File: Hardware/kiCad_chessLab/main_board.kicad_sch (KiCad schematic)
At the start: 23 parts, among them IC4 ESP32-C6-WROOM-1-N8, J4 TYPE-C-31-M-12, J5 DATA, J6 PWR, SW2 RST, SW3 BOOT, U3 74HC138

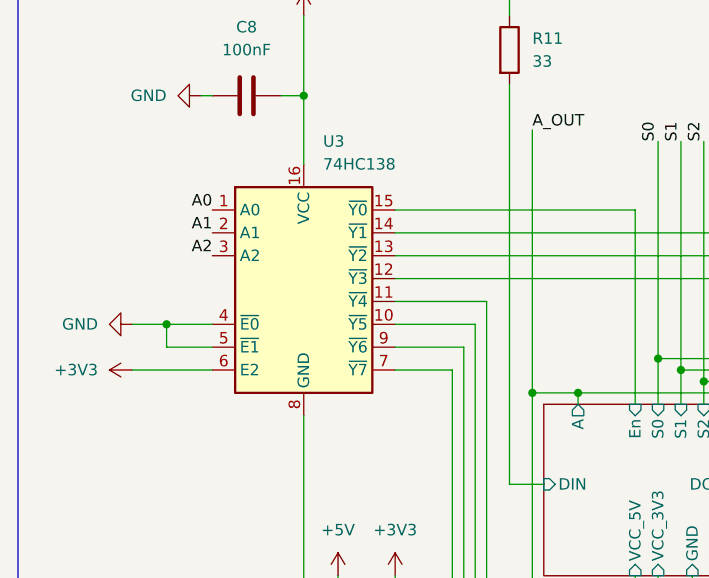
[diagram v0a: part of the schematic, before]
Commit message: NEW REFERENCES
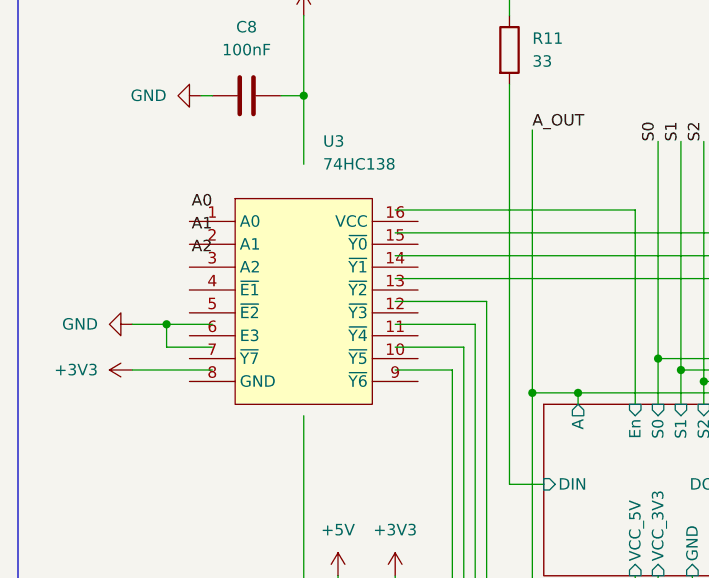
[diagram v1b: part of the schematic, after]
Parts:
- U3: footprint Package_SO:SOIC-16_3.9x9.9mm_P1.27mm -> chessLab-footprints:SOIC-16_L9.9-W3.9-P1.27-LS6.0-BL; symbol 74xx:74HC138 -> chessLab-symbols:74HC138D,653
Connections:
- net +3V3: no longer U3.16 (VCC), U3.6 (E2)
- net A0: no longer U3.1 (A0)
- net A1: no longer U3.2 (A1)
- net A2: no longer U3.3 (A2)
- net GND: no longer U3.4 (~{E0}), U3.5 (~{E1}), U3.8 (GND)
- net Row_A/En: no longer U3.15 (~{Y0})
- net Row_B/En: no longer U3.14 (~{Y1})
- net Row_C/En: no longer U3.13 (~{Y2})
- net Row_D/En: no longer U3.12 (~{Y3})
- net Row_E/En: no longer U3.11 (~{Y4})
- net Row_F/En: no longer U3.10 (~{Y5})
- net Row_G/En: no longer U3.9 (~{Y6})
- net Row_H/En: no longer U3.7 (~{Y7})
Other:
- moved on the sheet: U3
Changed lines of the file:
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@@
 	)
 	(symbol
-		(lib_id "74xx:74HC138")
+		(lib_id "chessLab-symbols:74HC138D,653")
 		(at 45.72 57.15 0)
 		(unit 1)
@@
 			)
 		)
-		(property "Footprint" "Package_SO:SOIC-16_3.9x9.9mm_P1.27mm"
+		(property "Footprint" "chessLab-footprints:SOIC-16_L9.9-W3.9-P1.27-LS6.0-BL"
 			(at 45.72 57.15 0)
 			(hide yes)

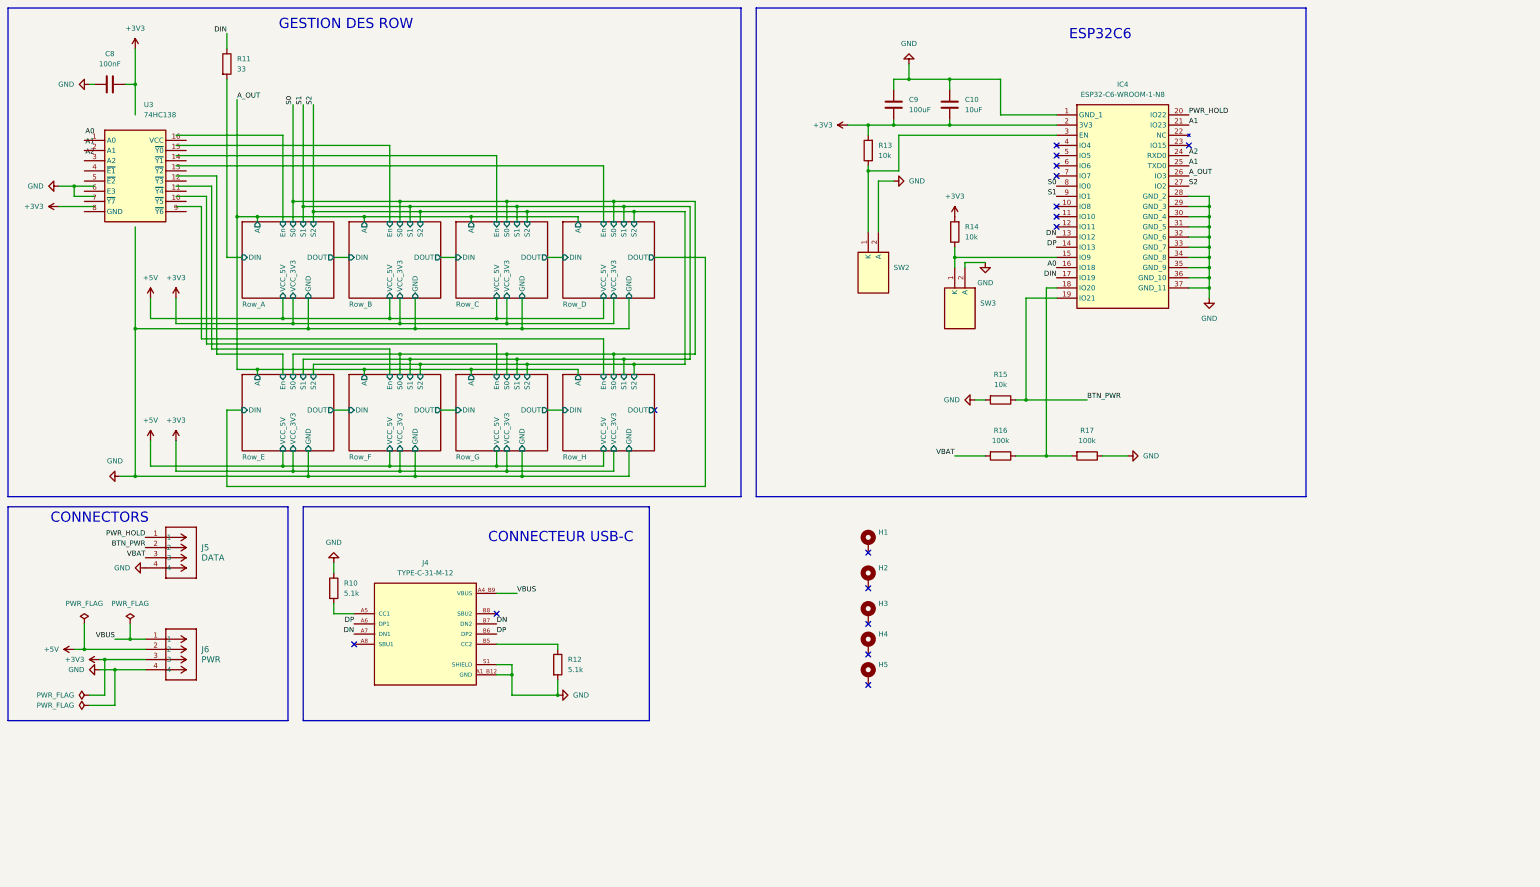
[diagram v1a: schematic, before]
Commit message: Usb c new design
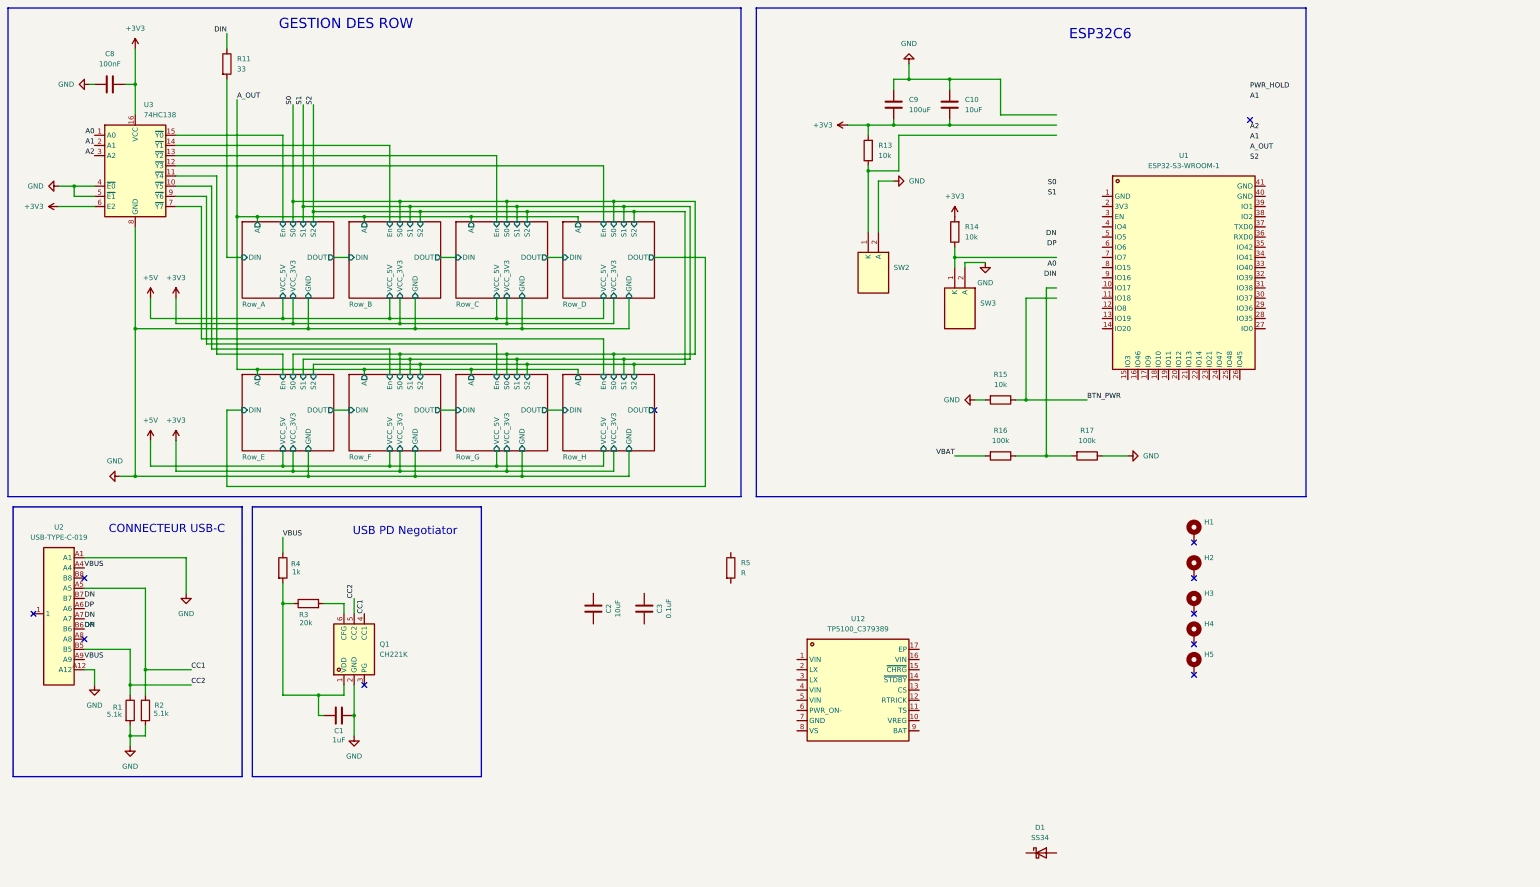
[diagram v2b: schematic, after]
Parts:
- removed IC4: ESP32-C6-WROOM-1-N8, chessLab-footprints:ESP32C6WROOM1N8, symbol chessLab-symbols:ESP32-C6-WROOM-1-N8
- removed J4: TYPE-C-31-M-12, chessLab-footprints:HRO_TYPE-C-31-M-12, symbol chessLab-symbols:TYPE-C-31-M-12
- removed J5: DATA, Connector_JST:JST_XH_B4B-XH-A_1x04_P2.50mm_Vertical, symbol chessLab-symbols:1048
- removed J6: PWR, Connector_JST:JST_XH_B4B-XH-A_1x04_P2.50mm_Vertical, symbol chessLab-symbols:1048
- removed R10, R12: 5.1k, Resistor_SMD:R_0603_1608Metric_Pad0.98x0.95mm_HandSolder, symbol Device:R
- added C1: 1uF, Capacitor_SMD:C_0201_0603Metric_Pad0.64x0.40mm_HandSolder, symbol Device:C
- added C2: 10uF, Capacitor_SMD:C_0201_0603Metric_Pad0.64x0.40mm_HandSolder, symbol Device:C
- added C3: 0.1uF, Capacitor_SMD:C_0201_0603Metric_Pad0.64x0.40mm_HandSolder, symbol Device:C
- added D1: SS34, Diode_SMD:D_SMA_Handsoldering, symbol Diode:SS34
- added Q1: CH221K, chessLab-footprints:SOT-23-6_L2.9-W1.6-P0.95-LS2.8-BL-2, symbol chessLab-symbols:CH221K
- added R1, R2: 5.1k, Resistor_SMD:R_0603_1608Metric_Pad0.98x0.95mm_HandSolder, symbol Device:R
- added R3: 20k, Resistor_SMD:R_0603_1608Metric_Pad0.98x0.95mm_HandSolder, symbol Device:R
- added R4: 1k, Resistor_SMD:R_0603_1608Metric_Pad0.98x0.95mm_HandSolder, symbol Device:R
- added R5: R, Resistor_SMD:R_0603_1608Metric_Pad0.98x0.95mm_HandSolder, symbol Device:R
- added U1: ESP32-S3-WROOM-1, chessLab-footprints:WIRELM-SMD_ESP32-S3-WROOM-1, symbol chessLab-symbols:ESP32-S3-WROOM-1
- added U12: TP5100_C379389, chessLab-footprints:TQFN-16_L4.0-W4.0-P0.65-BL-EP, symbol chessLab-symbols:TP5100_C379389
- added U2: USB-TYPE-C-019, chessLab-footprints:TYPE-C-SMD_HX-TYPE-C-16PIN, symbol chessLab-symbols:USB-TYPE-C-019
- U3: footprint chessLab-footprints:SOIC-16_L9.9-W3.9-P1.27-LS6.0-BL -> Package_SO:SOIC-16_3.9x9.9mm_P1.27mm; symbol chessLab-symbols:74HC138D,653 -> 74xx:74HC138
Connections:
- net +3V3: now also U3.16 (VCC), U3.6 (E2)
- net A0: now also U3.1 (A0)
- net A1: now also U3.2 (A1)
- net A2: now also U3.3 (A2)
- net DN: now also U2.A6, U2.A7, U2.B6, U2.B7
- net GND: now also U3.4 (~{E0}), U3.5 (~{E1}), U3.8 (GND), C1.2, Q1.2 (GND), R1.2, R2.2, U2.A1, U2.A12
- net Row_A/En: now also U3.15 (~{Y0})
- net Row_B/En: now also U3.14 (~{Y1})
- net Row_C/En: now also U3.13 (~{Y2})
- net Row_D/En: now also U3.12 (~{Y3})
- net Row_E/En: now also U3.11 (~{Y4})
- net Row_F/En: now also U3.10 (~{Y5})
- net Row_G/En: now also U3.9 (~{Y6})
- net Row_H/En: now also U3.7 (~{Y7})
- net VBUS: now also R4.1, U2.A4, U2.A9
- new net: C1.1, Q1.1 (VDD), R3.1, R4.2
- new net: Q1.6 (CFG), R3.2
- new net CC1: Q1.4 (CC1), R2.1, U2.A5
- new net CC2: Q1.5 (CC2), R1.1, U2.B5
- no-connect marks 16 -> 11
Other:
- note added: "USB PD Negotiator"
- note removed: "CONNECTORS"
- moved on the sheet: H1, H2, H3, H4, H5, U3

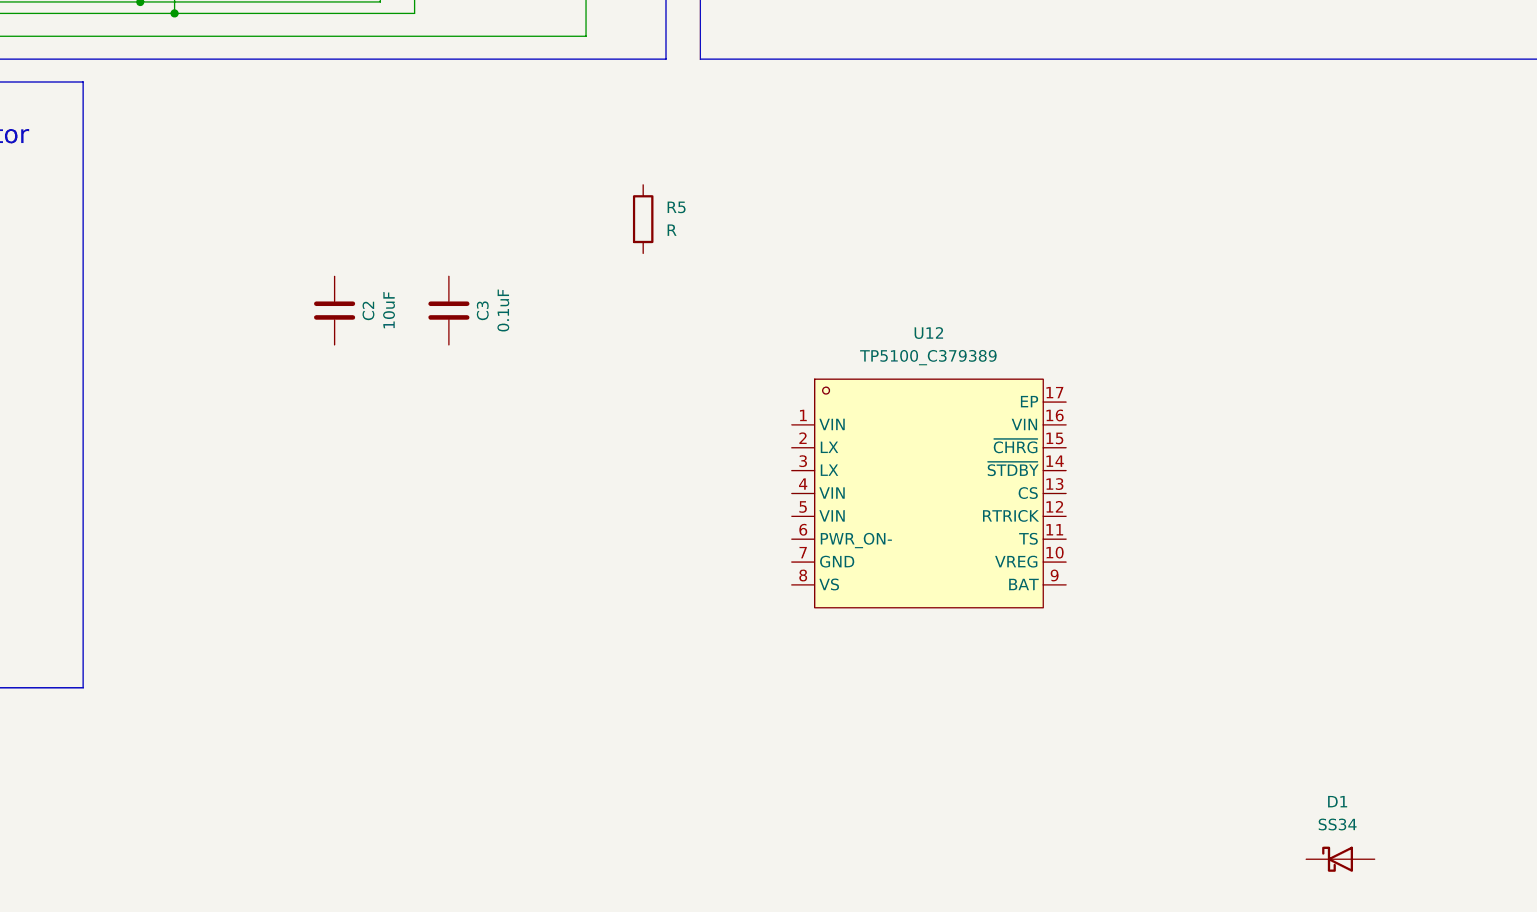
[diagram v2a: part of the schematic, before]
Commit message: avance
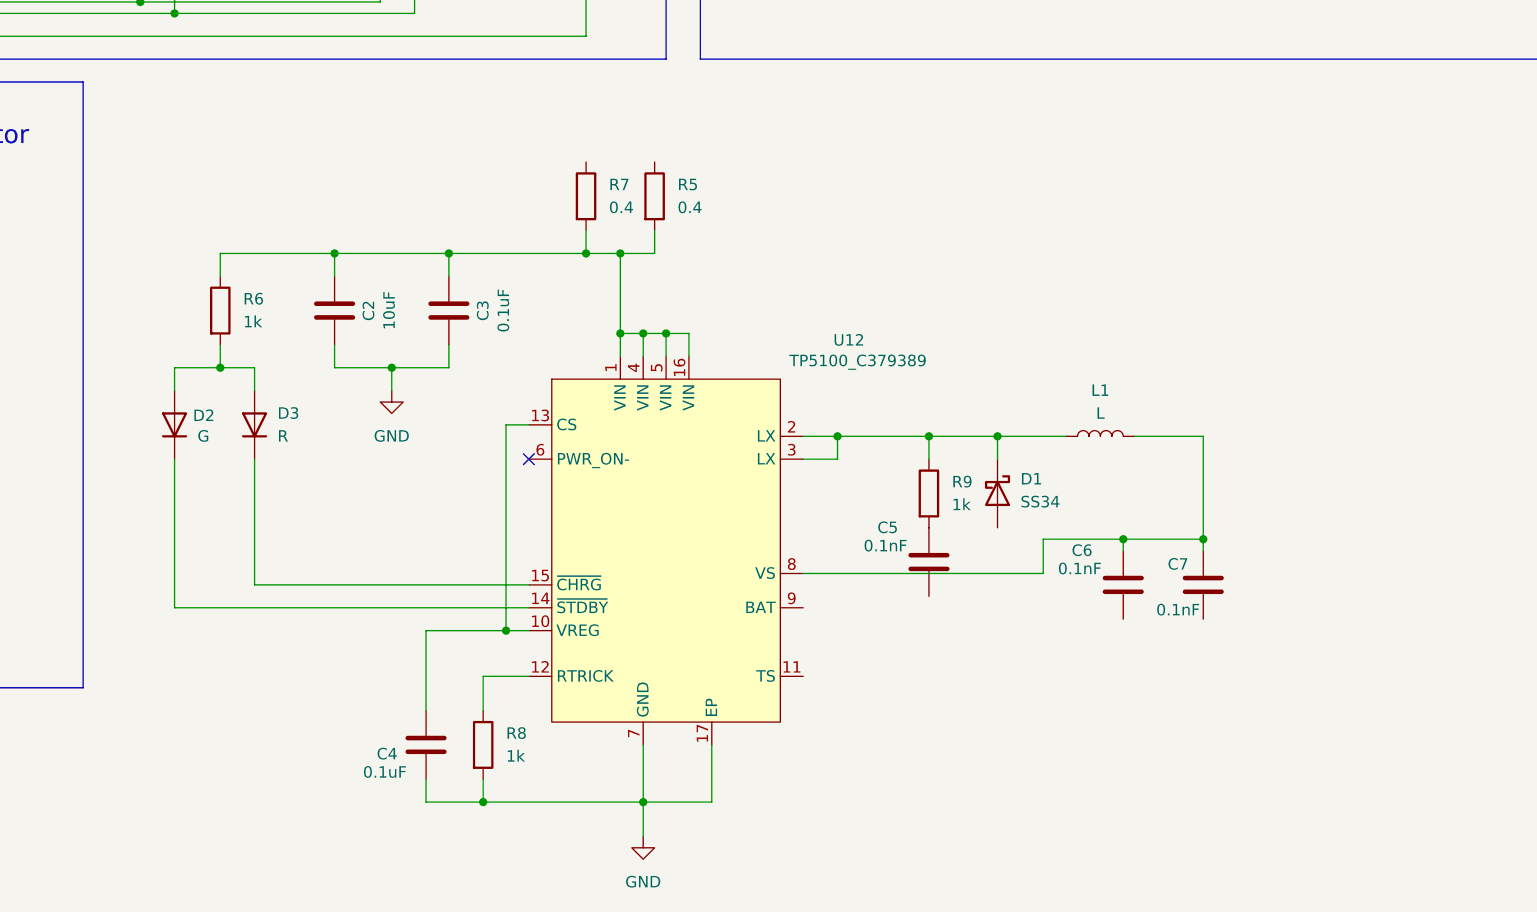
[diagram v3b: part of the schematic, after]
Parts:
- added C4: 0.1uF, Capacitor_SMD:C_0201_0603Metric_Pad0.64x0.40mm_HandSolder, symbol Device:C
- added C5, C6, C7: 0.1nF, Capacitor_SMD:C_0201_0603Metric_Pad0.64x0.40mm_HandSolder, symbol Device:C
- added D2: G, Diode_SMD:D_1206_3216Metric, symbol Device:D
- added D3: R, Diode_SMD:D_1206_3216Metric, symbol Device:D
- added L1: L, symbol Device:L
- added R6, R8, R9: 1k, Resistor_SMD:R_0603_1608Metric_Pad0.98x0.95mm_HandSolder, symbol Device:R
- added R7: 0.4, Resistor_SMD:R_1206_3216Metric_Pad1.30x1.75mm_HandSolder, symbol Device:R
- R5: value R -> 0.4; footprint Resistor_SMD:R_0603_1608Metric_Pad0.98x0.95mm_HandSolder -> Resistor_SMD:R_1206_3216Metric_Pad1.30x1.75mm_HandSolder
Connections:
- net GND: now also C2.1, C3.1, U12.17 (EP), U12.7 (GND), C4.1, R8.2
- net at R5.2: now also C2.2, C3.2, U12.1 (VIN), U12.16 (VIN), U12.4 (VIN), U12.5 (VIN), R6.1, R7.2
- net at U12.10 (VREG): now also U12.13 (CS), C4.2
- net at U12.12 (RTRICK): now also R8.1
- net at U12.14 (~{STDBY}): now also D2.1 (K)
- net at U12.15 (~{CHRG}): now also D3.1 (K)
- net at U12.2 (LX): now also D1.1 (K), U12.3 (LX), L1.1, R9.1
- net at U12.8 (VS): now also C6.2, C7.2, L1.2
- new net: D2.2 (A), D3.2 (A), R6.2
- new net: C5.2, R9.2
- no-connect marks 11 -> 12
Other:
- moved on the sheet: D1, R5
